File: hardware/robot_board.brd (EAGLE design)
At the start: 95.2 x 76.1 mm, 136 parts, among them J1 POWER_JACKPTH, Q1 DMP2035U, Q2 DMP2035U, Q3 DMP2035U-7, Q4 DMP2035U-7, U1 FT232RL-BASICSSOP, U11 LM393, U12 LM393, U16 LM393, U17 ATMEGA325PA, U2 SIA907EDJT, U3 MIC5219, U4 HC_05, U5 SIA907EDJT, U6 SIA907EDJT, U7 TLV70233, Y1 16MHz

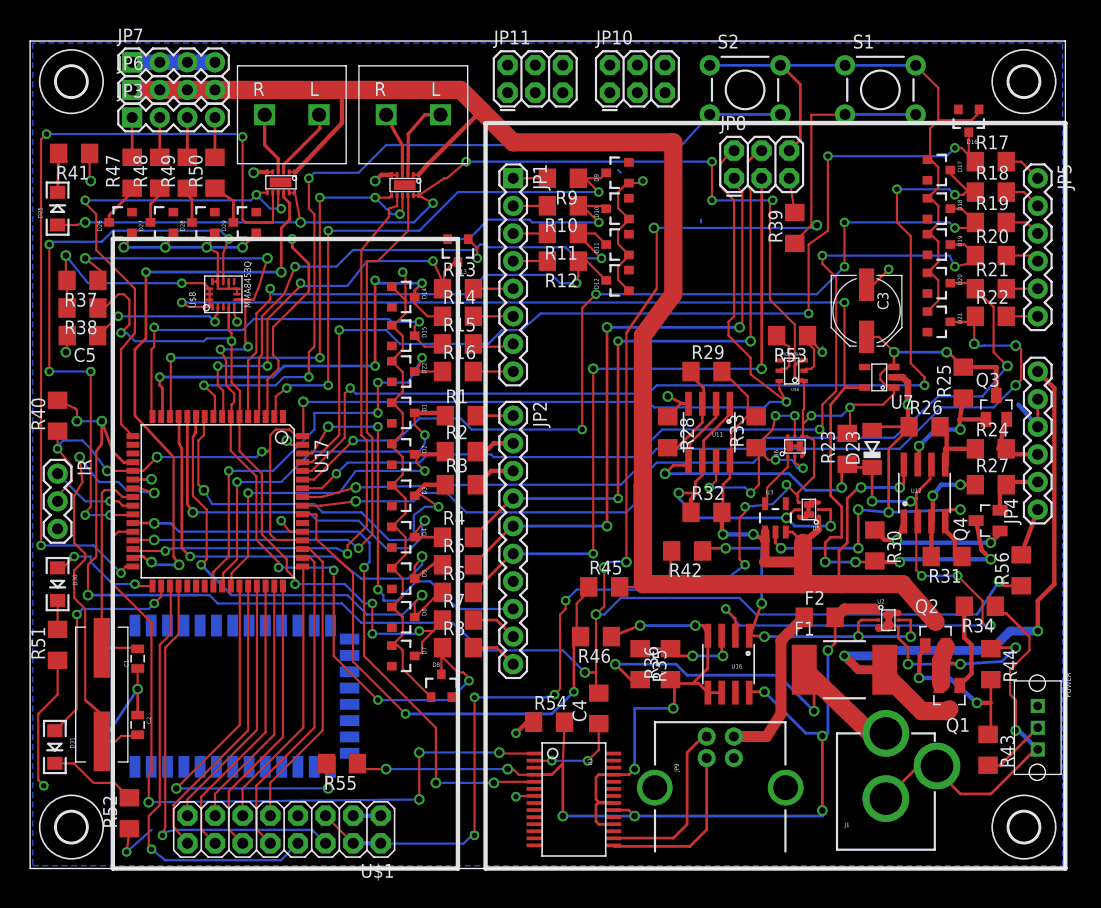
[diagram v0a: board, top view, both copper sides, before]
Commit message: updated bluetooth
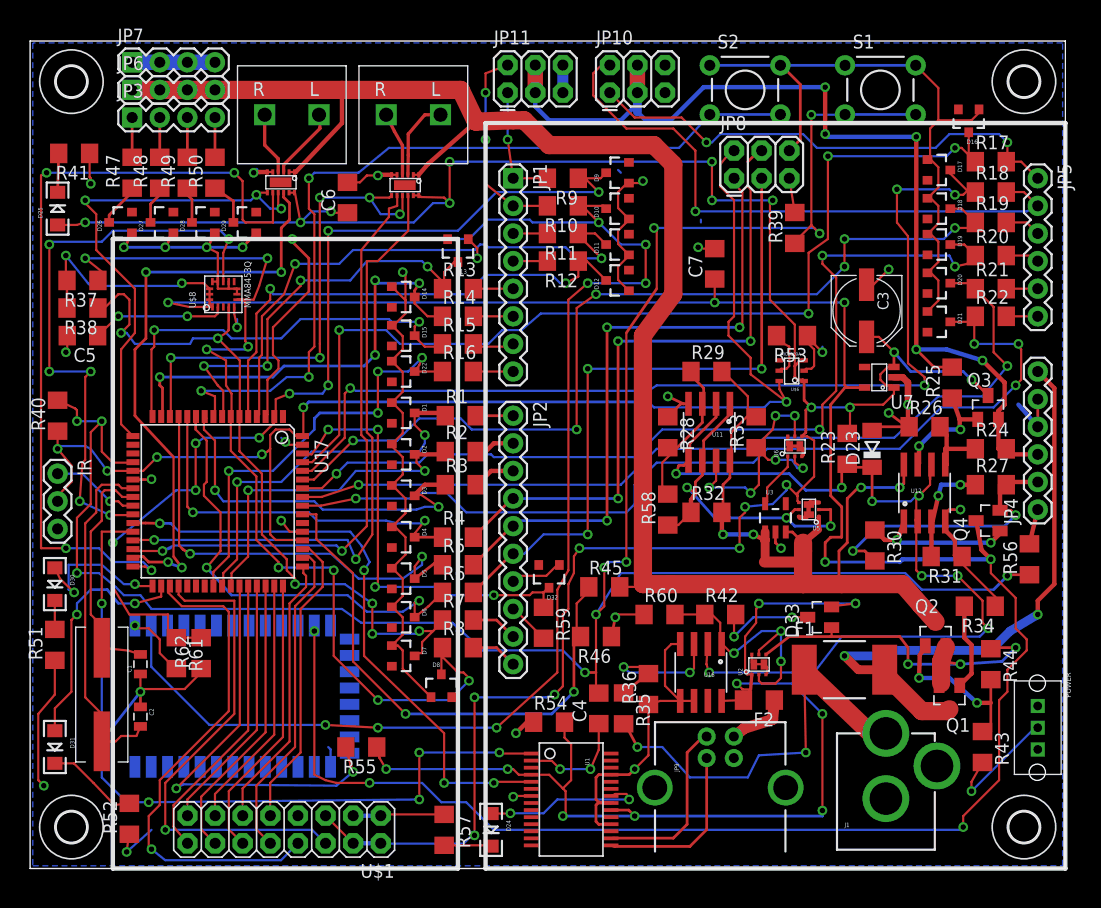
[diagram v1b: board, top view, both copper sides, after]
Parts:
- added C6: .1uF, resistor:C1206
- added C7: 22uF, resistor:C1206
- added D24: POWER, SparkFun-LED:LED-1206
- added D32: 5.1V, SparkFun-DiscreteSemi:SOT23-3
- added D33: BAT54C, diode:SOT23
- added R57: 330, resistor:R1206
- added R58, R60: 300K, resistor:R1206
- added R59, R61: 1K, resistor:R1206
- added R62: 2K, resistor:R1206
- R23, R27, R28, R35, R45, R46: value (none) -> 10K
- R24: value (none) -> 12K
- R26: value (none) -> 7.68K
- R29, R31: value (none) -> 15K
- R36: value (none) -> 20K
- moved U2 12.6 mm to (67.1, 18.8), turned to 0 degrees
- moved F2 9.45 mm to (67.1, 15.5), turned to 180 degrees
- moved R42 6.59 mm to (63.5, 23.4), turned to 0 degrees
- moved R35 4.34 mm to (54.6, 14.7)
- moved R36 3.06 mm to (56.9, 16.5)
- moved U16 2.65 mm to (61.7, 18.0)
- moved R55 2.34 mm to (30.5, 11.2)
- moved R56 1.27 mm to (91.9, 28.4)
- moved R25 1.02 mm to (84.8, 44.7)
- moved C2 0.80 mm to (10.2, 14.0)
- moved Q3 0.76 mm to (88.1, 42.4)
- moved R43 0.57 mm to (87.6, 11.2)
- moved C1 0.57 mm to (10.2, 18.8)
- moved R52 0.51 mm to (9.14, 4.57)
- moved D30 0.25 mm to (2.29, 26.2)
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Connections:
- removed net N$31: U$6.P$4
- new net AREF_IN: D32.3, R59.1, U17.62
- new net N$10: D24.A, U1.22
- new net N$11: D24.C, R57.2
- new net N$12: D33.3, R42.2
- new net N$14: R61.2, U4.1
- net 3V3: now also C7.1, U4.12; no longer R30.2
- net 3V3_OUT: now also R30.2
- net 5V: now also C6.1; no longer R25.2
- net 5VREG_SWO: now also R58.1
- net 5V_OUT: now also JP10.3, JP10.4, JP11.3, JP11.4, R25.2
- net A0: now also JP10.1
- net A1: now also JP10.2
- net AREF: now also R59.2; no longer U17.62
- net D0: now also JP11.1
- net D0_IN: now also R61.1, R62.2
- net D1: now also JP11.2
- net D1_IN: now also U4.2
- net GND: now also C6.2, C7.2, D32.1, JP10.5, JP10.6, JP11.5, JP11.6, R57.1, R60.1, R62.1, U4.13, U4.22
- net N$35: now also R58.2
- net PWR_SW: now also D33.1
- net USBGATE: now also R60.2
- net USB_5V: now also D33.2
- net VIN_F: no longer R42.2
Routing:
- net 3V3: track 135.0 -> 243.7 mm, vias 8 -> 10
- net D1_IN: track 53.4 -> 149.7 mm, vias 2 -> 8
- net 5V_OUT: track 6.95 -> 94.0 mm, vias 0 -> 5
- net A1: track 3.42 -> 56.0 mm, vias 0 -> 1
- net A0: track 3.53 -> 45.5 mm, vias 0 -> 2
- net AREF_IN: track 0.00 -> 40.7 mm, vias 0 -> 4
- net GND: track 357.9 -> 319.7 mm, vias 34 -> 30
- net D0_IN: track 53.0 -> 90.3 mm, vias 4 -> 8
- net AREF: track 38.4 -> 3.91 mm, vias 3 -> 0
- net 3V3_OUT: track 6.08 -> 26.5 mm, vias 0 -> 2
- net D1: track 3.15 -> 18.7 mm, vias 0 -> 2
- net N$10: track 0.00 -> 15.3 mm, vias 0 -> 2
- net PWR_SW: track 22.1 -> 34.9 mm
- net USB_5V: track 86.4 -> 98.3 mm, vias 8 -> 9
- net USBGATE: track 34.6 -> 23.3 mm, vias 5 -> 3
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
